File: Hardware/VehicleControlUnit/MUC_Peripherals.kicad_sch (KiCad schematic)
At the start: 0 parts

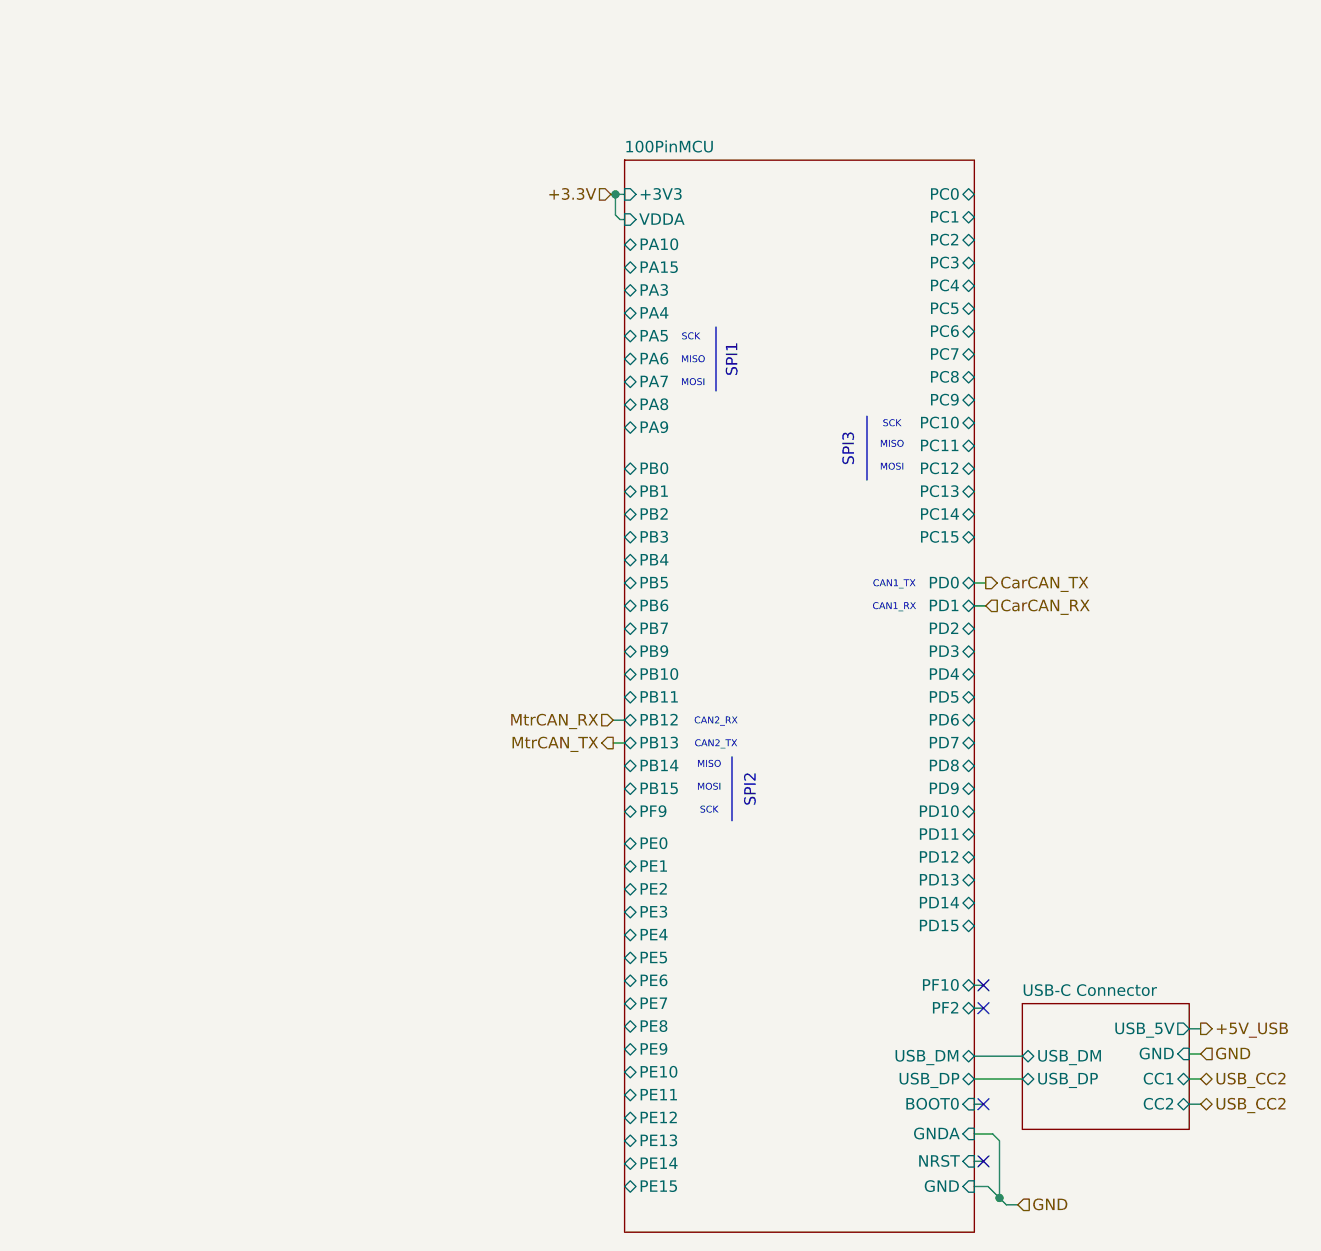
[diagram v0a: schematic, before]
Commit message: VCU more like diddle-u, mika time
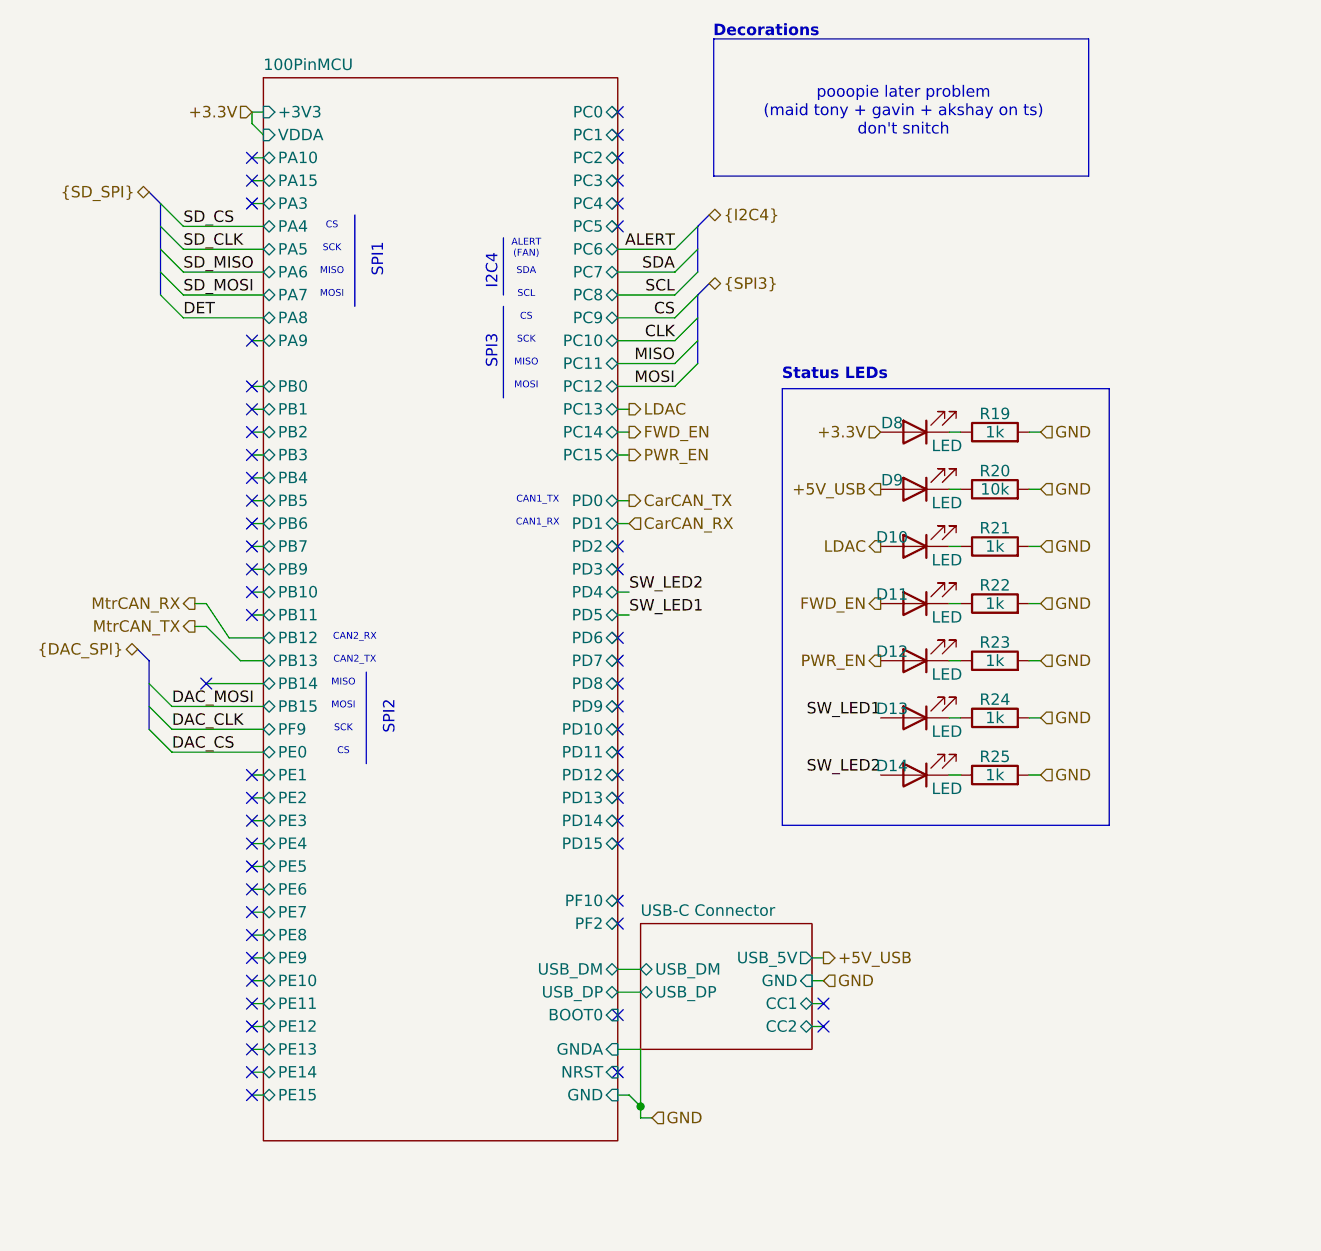
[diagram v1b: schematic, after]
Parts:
- added D10, D11, D12, D13, D14, D8, D9: LED, symbol Device:LED
- added R19, R21, R22, R23, R24, R25: 1k, symbol Device:R
- added R20: 10k, symbol Device:R
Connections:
- net +3.3V: now also D8.2 (A)
- net +5V_USB: now also D9.2 (A)
- net GND: now also R19.2, R20.2, R21.2, R22.2, R23.2, R24.2, R25.2
- new net: D12.1 (K), R23.1
- new net: D8.1 (K), R19.1
- new net: D9.1 (K), R20.1
- new net: D10.1 (K), R21.1
- new net: D11.1 (K), R22.1
- new net: D14.1 (K), R25.1
- new net: D13.1 (K), R24.1
- new net FWD_EN: D11.2 (A)
- new net LDAC: D10.2 (A)
- new net PWR_EN: D12.2 (A)
- new net SW_LED1: D13.2 (A)
- new net SW_LED2: D14.2 (A)
- no-connect marks 4 -> 55
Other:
- note added: "ALERT (FAN)"
- note added: "CS"
- note added: "Decorations"
- note added: "I2C4"
- note added: "SCL"
- note added: "SDA"
- note added: "Status LEDs"
- note added: "pooopie later problem (maid tony + gavin + akshay on ts) don't snitch"
